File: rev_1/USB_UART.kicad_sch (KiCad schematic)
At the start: 14 parts, among them J8 USB_B_Micro, U4 FT2232D, Y2 6MHz

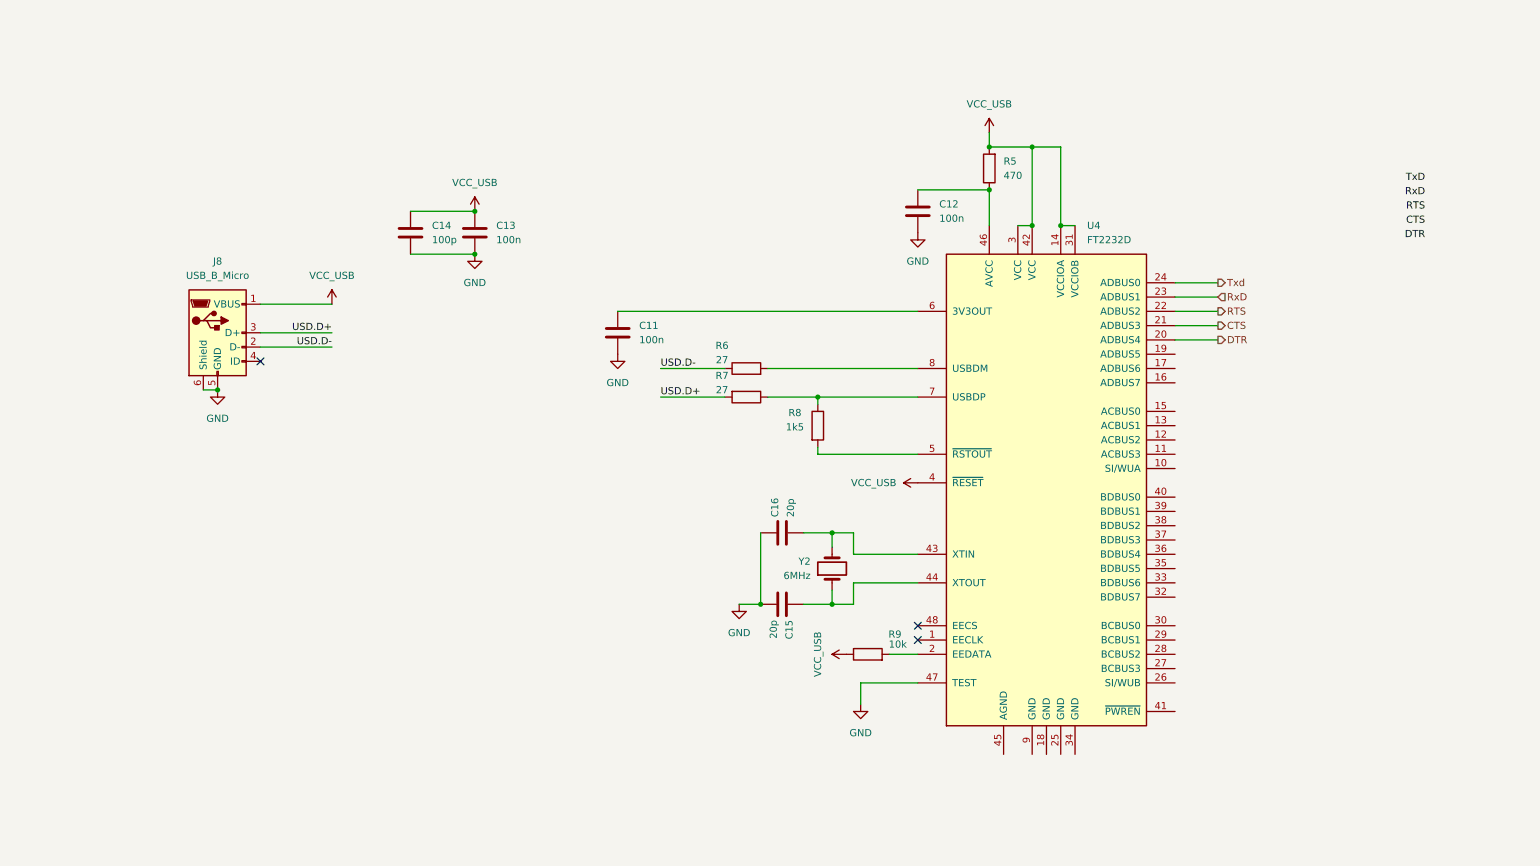
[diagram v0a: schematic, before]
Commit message: documentation
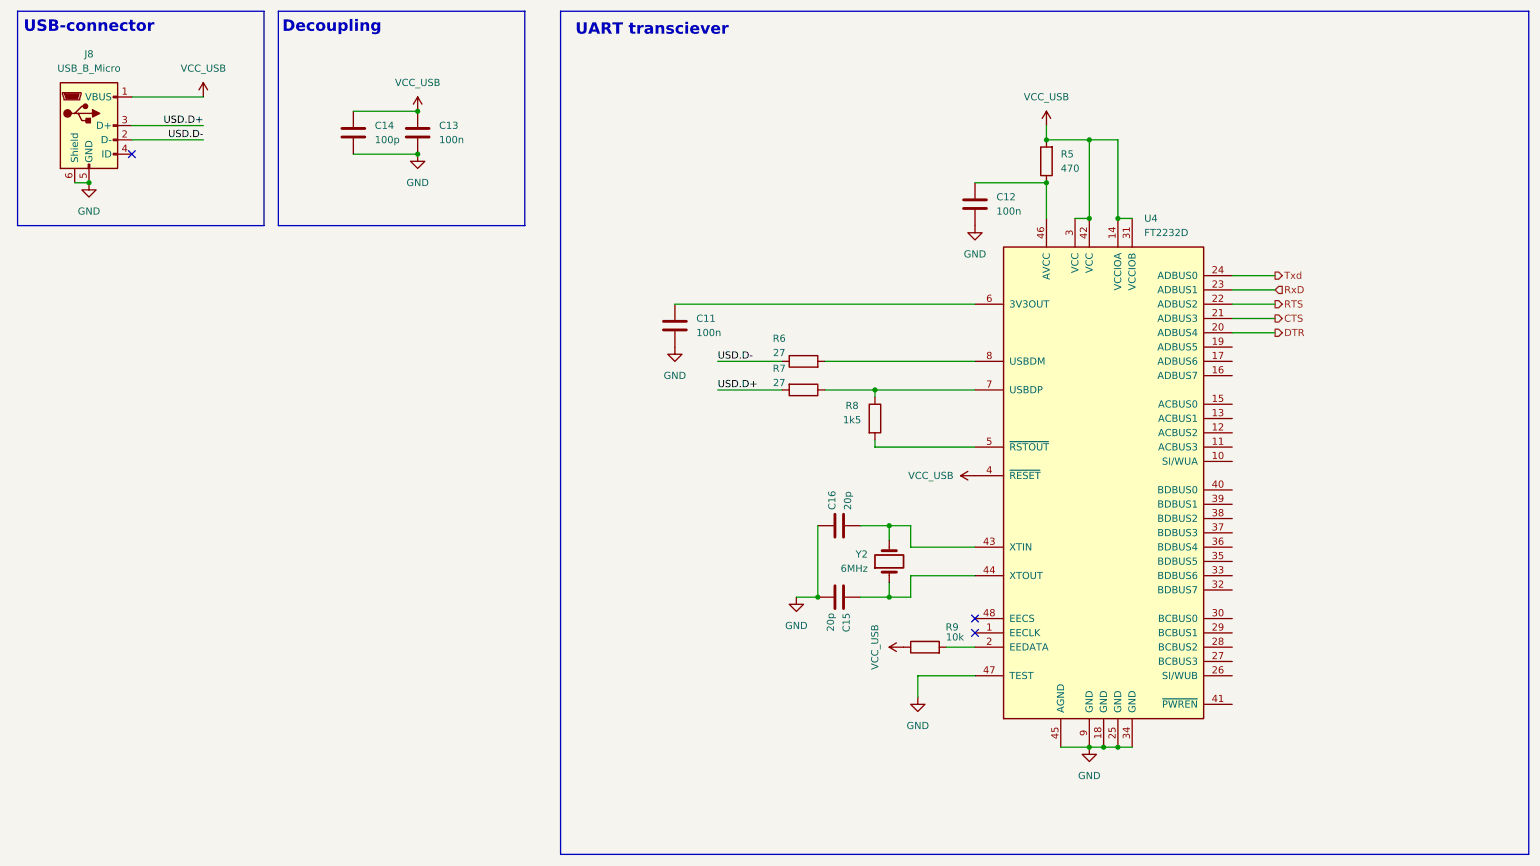
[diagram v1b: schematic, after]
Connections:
- net GND: now also U4.18 (GND), U4.25 (GND), U4.34 (GND), U4.45 (AGND), U4.9 (GND)
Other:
- note added: "Decoupling"
- note added: "UART transciever"
- note added: "USB-connector"
- title: (none) -> Beerduino
- moved on the sheet: C11, C12, C13, C14, C15, C16, J8, R5, R6, R7, R8, R9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
